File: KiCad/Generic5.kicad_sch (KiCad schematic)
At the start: 22 parts, among them J2 Conn_01x04, J3 USB-C, U1 ESP32-PICO-MINI-02, U2 FT231XQ, U3 LMR16006+FB

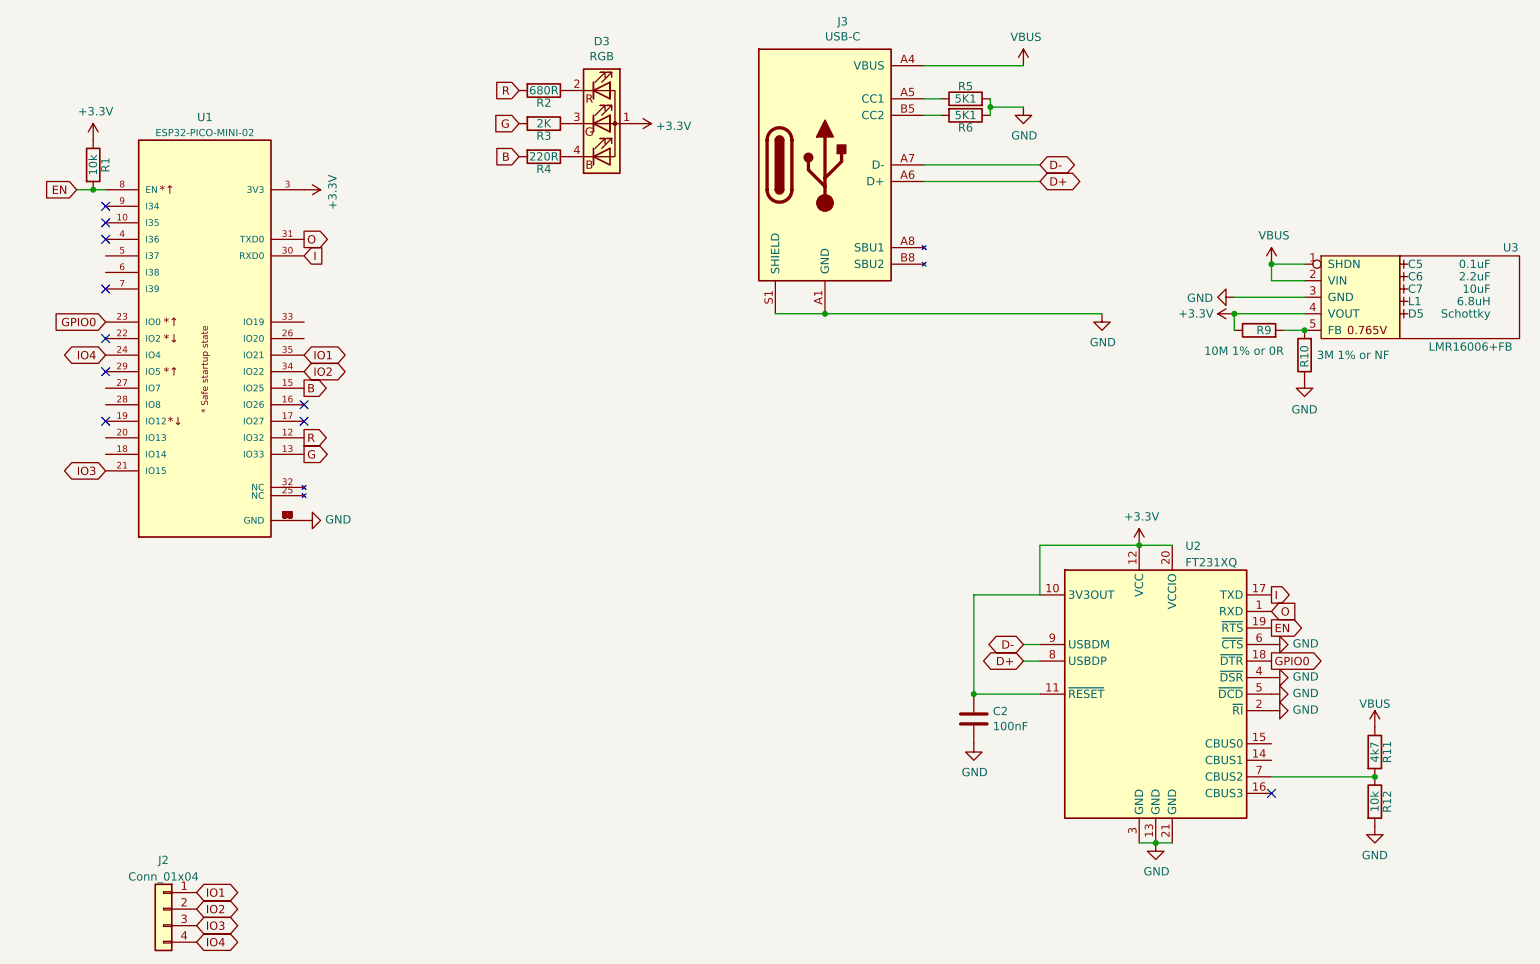
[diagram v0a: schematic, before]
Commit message: New Generic5
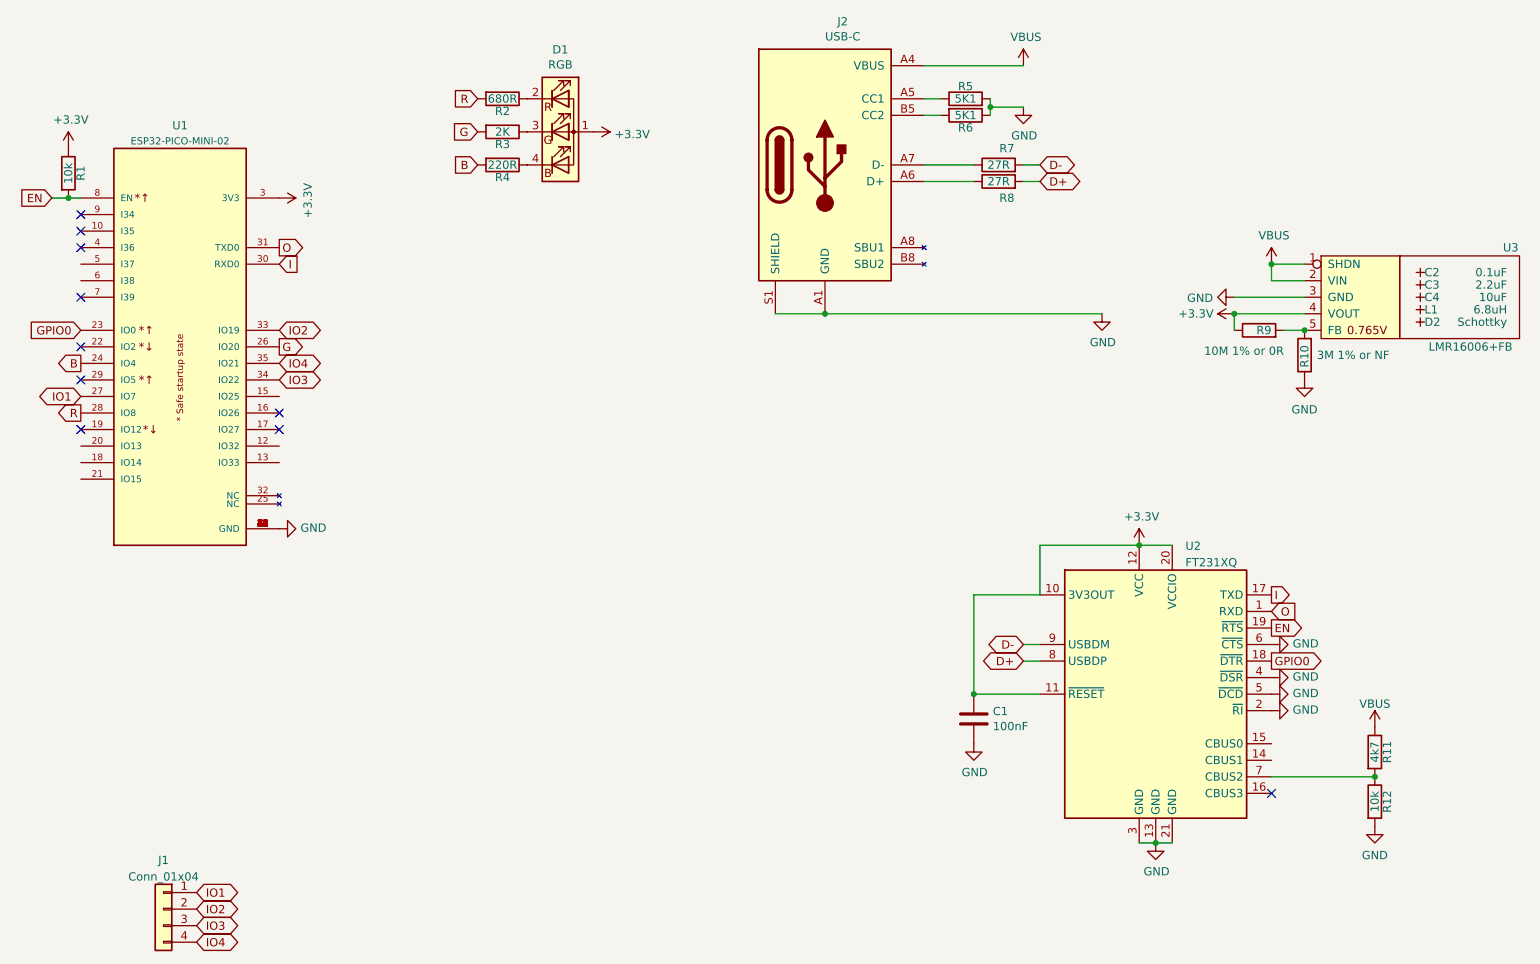
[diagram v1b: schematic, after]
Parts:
- added R7, R8: 27R, RevK:R_0603, symbol Device:R
- renumbered C2 to C1, C5 to C2, C6 to C3, C7 to C4, D3 to D1, D5 to D2, J2 to J1, J3 to J2
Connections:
- net B: now also U1.24 (IO4); no longer U1.15 (IO25)
- net D+: now also R8.2; no longer J2.A6 (D+), J2.B6 (D+)
- net D-: now also R7.2; no longer J2.A7 (D-), J2.B7 (D-)
- net G: now also U1.26 (IO20); no longer U1.13 (IO33)
- net IO1: now also U1.27 (IO7); no longer U1.35 (IO21)
- net IO2: now also U1.33 (IO19); no longer U1.34 (IO22)
- net IO3: now also U1.34 (IO22); no longer U1.21 (IO15)
- net IO4: now also U1.35 (IO21); no longer U1.24 (IO4)
- net R: now also U1.28 (IO8); no longer U1.12 (IO32)
- new net: J2.A6 (D+), J2.B6 (D+), R8.1
- new net: J2.A7 (D-), J2.B7 (D-), R7.1
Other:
- moved on the sheet: C2, C3, C4, D1, D2, L1, R1, R2, R3, R4, U1
